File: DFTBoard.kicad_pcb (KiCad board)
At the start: 8 copper layers, 148.5 x 62 mm, 76 parts, among them CON1 AVR-JTAG-10, CON2 AVR-JTAG-10, J1 AUDIO JACK, J2 JACK_TRS_4PINS, J3 AUDIO JACK, J4 AUDIO JACK, J5 USB_A, J6 Micro_SD_Card_Det, SW1 TL6215RF200BDT, U10 APDS-9960, U11 W9751G6KB, U12 W9751G6KB, U7 TLV320AIC3104, U9 VL53L0X

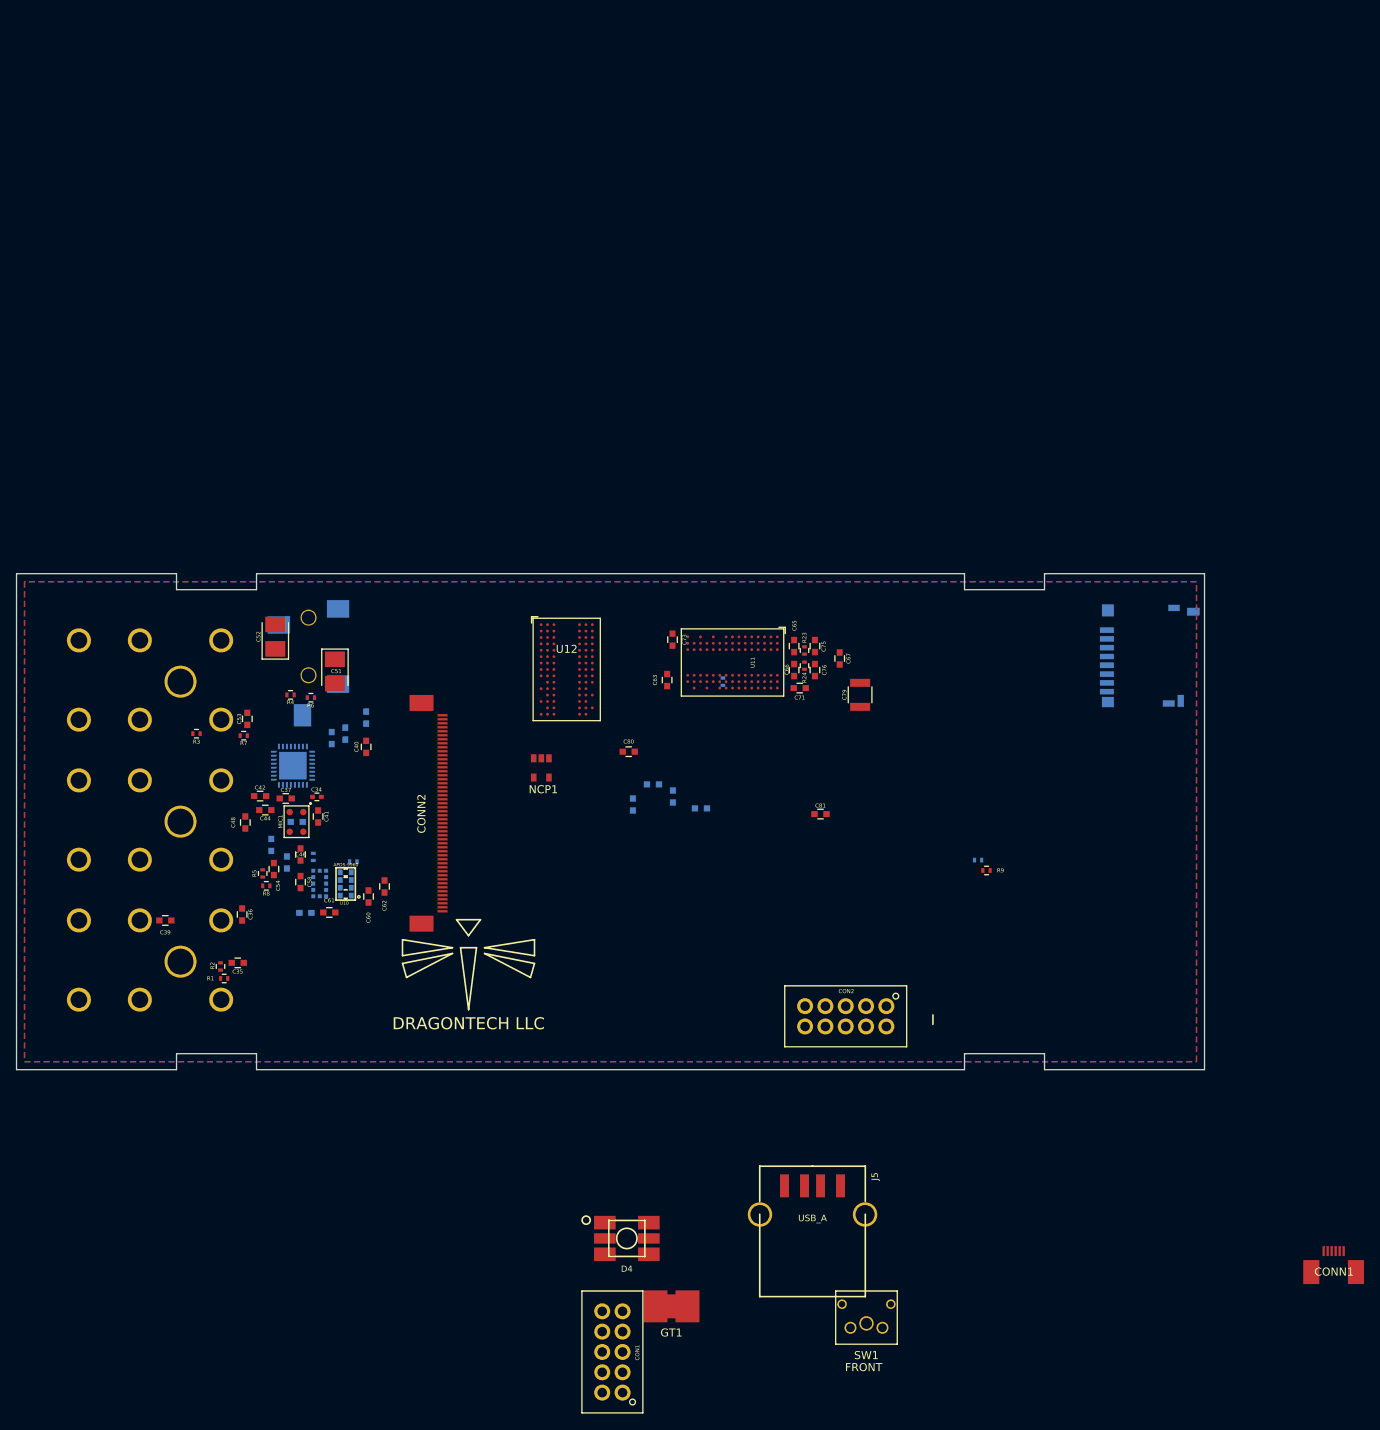
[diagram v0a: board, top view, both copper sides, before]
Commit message: passes ERC, about to update footprints to v5 references
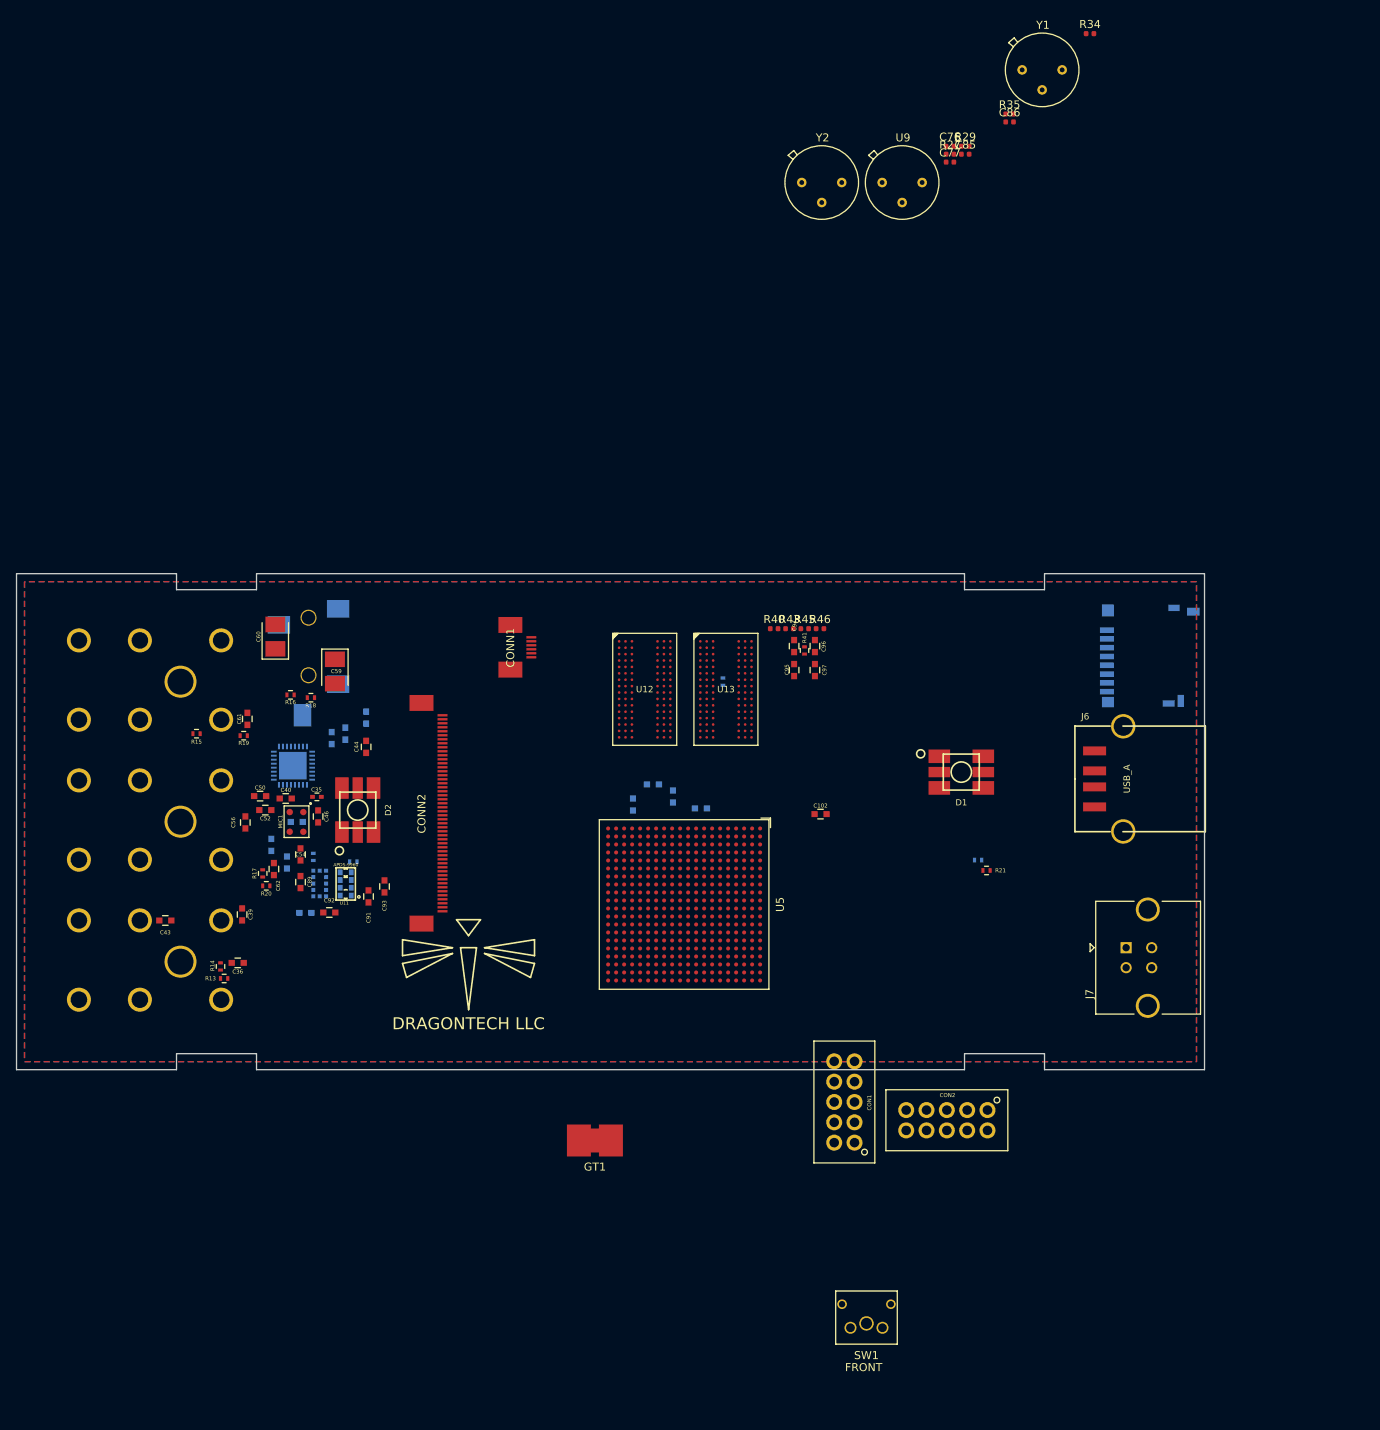
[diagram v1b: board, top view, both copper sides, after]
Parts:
- removed C63, C67: 10uF, Capacitors_SMD:C_0603
- removed C71, C73: .1uF, Capacitors_SMD:C_0603
- removed C79: 47uF, Capacitors_SMD:C_1210
- removed C80: 4.7uF, Capacitors_SMD:C_0603
- removed D4: LED_RGB, DFTcustom:PLCC6-SM-RGB-LED
- removed NCP1: NCP361, DFTcustom:TSOP-5
- removed R24: 10k, Resistors_SMD:R_0402
- removed the U11 at (196.0, 104.1)
- added C76: 18pF, Capacitor_SMD:C_0402_1005Metric, F.Cu at (223.2, 39.6)
- added C77: 18pF, Capacitor_SMD:C_0402_1005Metric, F.Cu at (223.2, 41.6)
- added C85: 18pF, Capacitor_SMD:C_0402_1005Metric, F.Cu at (225.1, 40.6)
- added C86: 18pF, Capacitor_SMD:C_0402_1005Metric, F.Cu at (230.6, 36.5)
- added D1: LED_RGB, DFTcustom:PLCC6-SM-RGB-LED, F.Cu at (224.6, 117.8)
- added D2: LED_RGB, DFTcustom:PLCC6-SM-RGB-LED, F.Cu at (149.2, 122.5)
- added J7: USB_B, Connector_USB:USB_B_Amphenol_MUSB-D511_Vertical_Rugged, F.Cu at (245.2, 139.8)
- added R27: 1M, Resistor_SMD:R_0402_1005Metric, F.Cu at (223.2, 40.6)
- added R29: 8.06k 1%, Resistor_SMD:R_0402_1005Metric, F.Cu at (225.1, 39.6)
- added R34: 1M, Resistor_SMD:R_0402_1005Metric, F.Cu at (240.7, 25.5)
- added R35: 8.06k 1%, Resistor_SMD:R_0402_1005Metric, F.Cu at (230.6, 35.5)
- added R40: 240 1%, Resistor_SMD:R_0402_1005Metric, F.Cu at (201.2, 99.9)
- added R43: 240 1%, Resistor_SMD:R_0402_1005Metric, F.Cu at (203.1, 99.9)
- added R45: 80.6, Resistor_SMD:R_0402_1005Metric, F.Cu at (205.0, 99.9)
- added R46: 80.6, Resistor_SMD:R_0402_1005Metric, F.Cu at (206.9, 99.9)
- added U13: MT41K256M16HA-125_E, DFTcustom:FBGA-96-DDR3-SDRAM, F.Cu at (195.2, 107.5)
- added U5: xc7z020clg400, Package_BGA:BGA-400_21.0x21.0mm_Layout20x20_P1.0mm, F.Cu at (189.9, 134.3)
- added U9: MIC2025-1YMM, Crystal:Crystal_HC35-U, F.Cu at (214.7, 44.1)
- added Y1: Crystal, Crystal:Crystal_HC35-U, F.Cu at (232.2, 30.0)
- added Y2: Crystal, Crystal:Crystal_HC35-U, F.Cu at (204.7, 44.1)
- R41: renamed from R23; value 10k -> 10k 1%
- U12: value W9751G6KB -> MT41K256M16HA-125_E; footprint DFTcustom:WBGA-84 -> DFTcustom:FBGA-96-DDR3-SDRAM
- moved CONN1 125.5 mm to (170.8, 102.2), turned to 270 degrees
- moved J6 63.9 mm to (242.7, 118.7), turned to 90 degrees
- moved CON1 42.6 mm to (211.2, 156.5)
- moved GT1 22.8 mm to (178.8, 163.8)
- moved CON2 18.1 mm to (220.2, 160.1)
- moved U12 10.1 mm to (185.0, 107.5)
- renumbered C81 to C102, C82 to C104, C83 to C105, C84 to C106, C85 to C107, C34 to C35, C35 to C36, C36 to C39, C37 to C40, C38 to C41, C39 to C43, C40 to C44, C41 to C46, C42 to C50, C43 to C51, C44 to C52, C45 to C53, C46 to C54, C47 to C55, C48 to C56, C49 to C57, C50 to C58, C51 to C59, C52 to C60, C53 to C61, C54 to C62, C58 to C89, C59 to C90, C60 to C91, C61 to C92, C62 to C93, C65 to C94, C66 to C95, C75 to C96, C76 to C97, J6 to J5, J5 to J6, R1 to R13, R2 to R14, R3 to R15, R4 to R16, R5 to R17, R6 to R18, R7 to R19, R8 to R20, R9 to R21, R10 to R22, R19 to R36, R20 to R37, R27 to R44, U9 to U10, U10 to U11, U7 to U6
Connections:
- C102 pad 1: +1.8V -> Net-(C100-Pad1)
- C104 pad 1: +1.8V -> Net-(C100-Pad1)
- C105 pad 1: +1.8V -> Net-(C100-Pad1)
- C106 pad 1: +1.8V -> Net-(C100-Pad1)
- C107 pad 1: +1.8V -> Net-(C100-Pad1)
- C94 pad 1: +1.8V -> +1V35
- C96 pad 1: +1.8V -> +1V35
- CON1 pad 1: (no net) -> AX_TCLK
- CON1 pad 3: (no net) -> AX_TDO
- CON1 pad 5: (no net) -> AX_TMS
- CON1 pad 9: (no net) -> AX_TDI
- CONN2 pad 10: (no net) -> LCD_RST
- CONN2 pad 11: (no net) -> RGB_VSYNC
- CONN2 pad 12: (no net) -> RGB_HSYNC
- CONN2 pad 13: (no net) -> RGB_DOTCLK
- CONN2 pad 14: (no net) -> RGB_DE
- CONN2 pad 15: (no net) -> LCD_D17
- CONN2 pad 16: (no net) -> LCD_D16
- CONN2 pad 17: (no net) -> LCD_D15
- CONN2 pad 18: (no net) -> LCD_D14
- CONN2 pad 19: (no net) -> LCD_D13
- CONN2 pad 20: (no net) -> LCD_D12
- CONN2 pad 21: (no net) -> LCD_D11
- CONN2 pad 22: (no net) -> LCD_D10
- CONN2 pad 23: (no net) -> LCD_D9
- CONN2 pad 24: (no net) -> LCD_D8
- CONN2 pad 25: (no net) -> LCD_D7
- CONN2 pad 26: (no net) -> LCD_D6
- CONN2 pad 27: (no net) -> LCD_D5
- CONN2 pad 28: (no net) -> LCD_D4
- CONN2 pad 29: (no net) -> LCD_D3
- CONN2 pad 30: (no net) -> LCD_D2
- CONN2 pad 31: (no net) -> LCD_D1
- CONN2 pad 32: (no net) -> LCD_D0
- CONN2 pad 33: (no net) -> LCD_SDO
- CONN2 pad 34: (no net) -> LCD_SDI
- CONN2 pad 35: (no net) -> LCD_READ
- CONN2 pad 36: (no net) -> LCD_WRITE
- CONN2 pad 37: (no net) -> LCD_DorI
- CONN2 pad 38: (no net) -> LCD_CS
- CONN2 pad 39: (no net) -> LCD_TE
- CONN2 pad 6: (no net) -> LCD_IM0
- CONN2 pad 7: (no net) -> LCD_IM1
- CONN2 pad 8: (no net) -> LCD_IM2
- CONN2 pad 9: (no net) -> LCD_IM3
- J5 pad 1: (no net) -> SD_D2
- J5 pad 2: (no net) -> SD_D3
- J5 pad 3: (no net) -> SD_CMD
- J5 pad 5: (no net) -> SD_CLK
- J5 pad 7: (no net) -> SD_D0
- J5 pad 8: (no net) -> SD_D1
- J5 pad 9: (no net) -> SD_CD
- J6 pad 1: SPIUSB_VBUS -> (no net)
- R21 pad 1: I2C_SCLK -> I2C3v3_SCLK
- R21 pad 2: +1.8V -> +3V3
- R22 pad 1: I2C_SDIN -> I2C3v3_SDIN
- R22 pad 2: +1.8V -> +3V3
- R41 pad 1: +1.8V -> +1V35
- SW1 pad 2: (no net) -> TEMPO_SW
- U10 pad 10: I2C_SCLK -> (no net)
- U10 pad 9: I2C_SDIN -> (no net)
- U11 pad 1: I2C_SDIN -> (no net)
- U11 pad 2: (no net) -> RF2_IRQ
- U11 pad 7: I2C_SCLK -> (no net)
- U12 pad A1: +1.8V -> +1V35
- U12 pad A2: (no net) -> DDR3_DQ29
- U12 pad A3: GND -> DDR3_DQ31
- U12 pad A7: GND -> DDR3_DQ28
- U12 pad A8: (no net) -> +1V35
- U12 pad A9: +1.8V -> GND
- U12 pad B1: (no net) -> GND
- U12 pad B2: GND -> +1V35
- U12 pad B3: (no net) -> GND
- U12 pad B7: (no net) -> DDR3_DQS3_N
- U12 pad B8: GND -> DDR3_DQ30
- U12 pad B9: (no net) -> GND
- U12 pad C1: +1.8V -> +1V35
- U12 pad C2: (no net) -> DDR3_DQ27
- U12 pad C3: +1.8V -> DDR3_DQ25
- U12 pad C7: +1.8V -> DDR3_DQS3_P
- U12 pad C8: (no net) -> DDR3_DQ26
- U12 pad C9: +1.8V -> +1V35
- U12 pad D1: (no net) -> GND
- U12 pad D2: GND -> +1V35
- U12 pad D3: (no net) -> DDR3_DM3
- U12 pad D7: (no net) -> DDR3_DQ24
- U12 pad D9: (no net) -> +1V35
- U12 pad E1: +1.8V -> GND
- U12 pad E2: (no net) -> GND
- U12 pad E3: GND -> DDR3_DQ16
- U12 pad E7: GND -> DDR3_DM2
- U12 pad E8: (no net) -> GND
- U12 pad E9: +1.8V -> +1V35
- U12 pad F1: (no net) -> +1V35
- U12 pad F2: GND -> DDR3_DQ18
- U12 pad F3: (no net) -> DDR3_DQS2_P
- U12 pad F7: (no net) -> DDR3_DQ17
- U12 pad F8: GND -> DDR3_DQ19
- U12 pad F9: (no net) -> GND
- U12 pad G1: +1.8V -> GND
- U12 pad G2: (no net) -> DDR3_DQ22
- U12 pad G3: +1.8V -> DDR3_DQS2_N
- U12 pad G7: +1.8V -> +1V35
- U12 pad G8: (no net) -> GND
- U12 pad G9: +1.8V -> GND
- U12 pad H1: (no net) -> /DDR3/VREF
- U12 pad H2: GND -> +1V35
- U12 pad H3: (no net) -> DDR3_DQ20
- U12 pad H7: (no net) -> DDR3_DQ23
- U12 pad H8: GND -> DDR3_DQ21
- U12 pad H9: (no net) -> +1V35
- U12 pad J1: +1.8V -> (no net)
- U12 pad J2: /DDR3/VREF -> GND
- U12 pad J3: GND -> DDR3_RAS#
- U12 pad J7: GND -> DDR3_CK_P
- U12 pad J8: DDR3_CK_P -> GND
- U12 pad J9: +1.8V -> (no net)
- U12 pad K2: DDR3_CKE -> +1V35
- U12 pad K3: DDR3_WE# -> DDR3_CAS#
- U12 pad K7: DDR3_RAS# -> DDR3_CK_N
- U12 pad K8: DDR3_CK_N -> +1V35
- U12 pad K9: DDR3_ODT -> DDR3_CKE
- U12 pad L2: DDR3_BA0 -> DDR3_CS#
- U12 pad L3: DDR3_BA1 -> DDR3_WE#
- U12 pad L7: DDR3_CAS# -> DDR3_A10
- U12 pad L8: DDR3_CS -> Net-(R40-Pad1)
- U12 pad M2: DDR3_A10 -> DDR3_BA0
- U12 pad M3: DDR3_A1 -> DDR3_BA2
- U12 pad M7: DDR3_A2 -> (no net)
- U12 pad M8: DDR3_A0 -> /DDR3/VREF
- U12 pad M9: +1.8V -> GND
- U12 pad N1: GND -> +1V35
- U12 pad N3: DDR3_A5 -> DDR3_A0
- U12 pad N7: DDR3_A6 -> DDR3_A12
- U12 pad N8: DDR3_A4 -> DDR3_BA1
- U12 pad P2: DDR3_A7 -> DDR3_A5
- U12 pad P3: DDR3_A9 -> DDR3_A2
- U12 pad P7: DDR3_A11 -> DDR3_A1
- U12 pad P8: DDR3_A8 -> DDR3_A4
- U12 pad R1: +1.8V -> +1V35
- U12 pad R2: DDR3_A12 -> DDR3_A7
- U12 pad R3: (no net) -> DDR3_A9
- U12 pad R7: (no net) -> DDR3_A11
- U12 pad R8: (no net) -> DDR3_A6
- U6 pad 1: (no net) -> I2S_MCLK
- U6 pad 2: (no net) -> I2S_BCLK
- U6 pad 3: (no net) -> I2S_LRCLK
- U6 pad 4: (no net) -> I2S_DACSD
- U6 pad 5: (no net) -> I2S_ADCSD
